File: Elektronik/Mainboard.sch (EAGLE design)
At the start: 21 parts

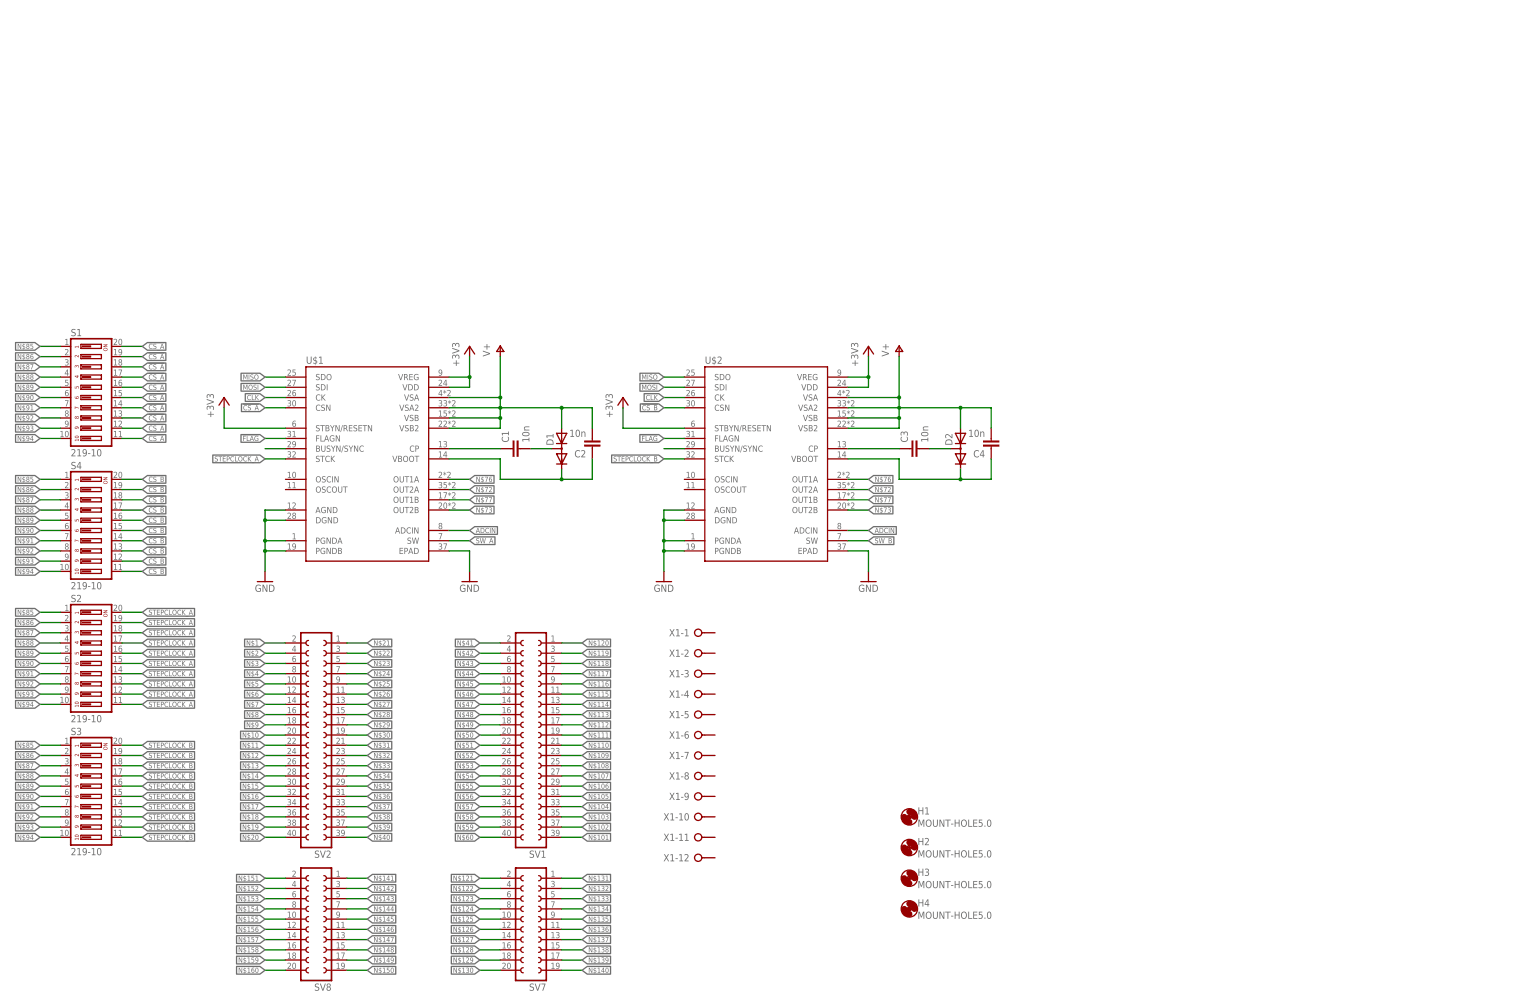
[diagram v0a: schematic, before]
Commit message: Elektronik auf den neusten Stand gebracht (Merge mit privater Dropbox
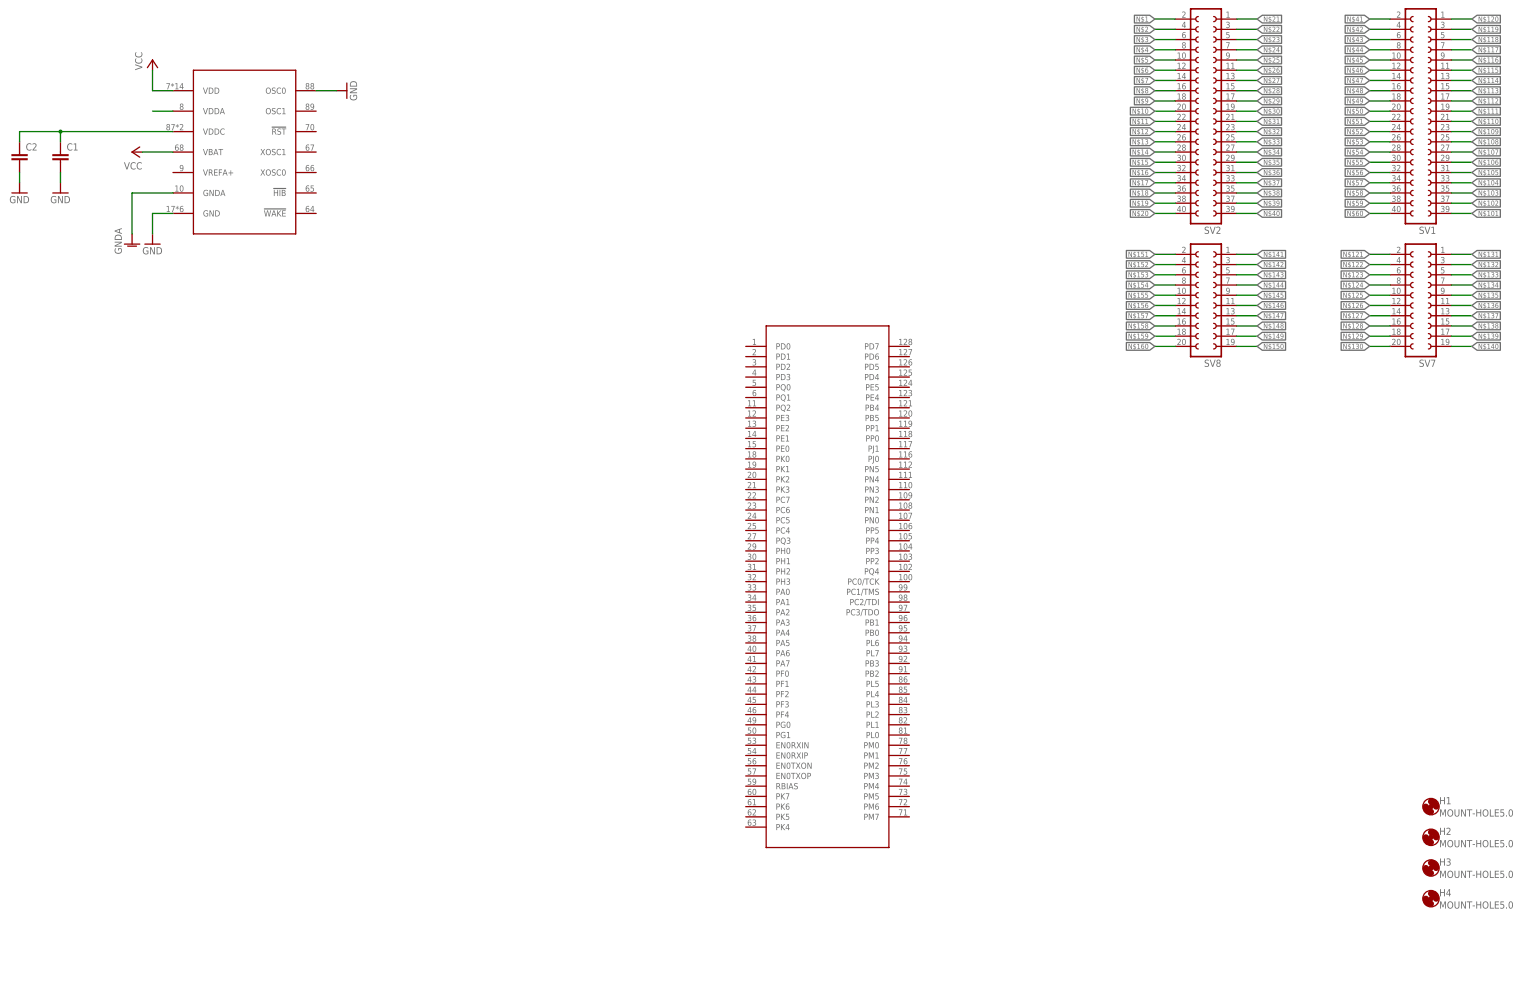
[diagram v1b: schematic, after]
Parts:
- removed C3, C4: 10n, rcl:C-EUC0805
- removed D1, D2: (no value), diode:DIODE_2CACA-SOT23
- removed S1, S2, S3, S4: 219-10, switch-dil:219-10
- removed U$2: L6470HPOWERSO36, Hardware:L6470HPOWERSO36
- removed X1: (no value), con-wago-508:W237-12P
- C1, C2: value 10n -> (none)
- U$1: value L6470HPOWERSO36 -> TM4C1294KCPDT; device Hardware:L6470HPOWERSO36 -> Hardware:TM4C1294KCPDT
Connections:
- removed net !CS_A: S1.11, S1.12, S1.13, S1.14, S1.15, S1.16, S1.17, S1.18, S1.19, S1.20, U$1.CSN
- removed net !CS_B: S4.11, S4.12, S4.13, S4.14, S4.15, S4.16, S4.17, S4.18, S4.19, S4.20, U$2.CSN
- removed net !FLAG: U$1.FLAGN, U$2.FLAGN
- removed net +3V3: U$1.STBYN/RESETN, U$1.VDD, U$1.VREG, U$2.STBYN/RESETN, U$2.VDD, U$2.VREG
- removed net ADCIN: U$1.ADCIN, U$2.ADCIN
- removed net CLK: U$1.CK, U$2.CK
- removed net MISO: U$1.SDO, U$2.SDO
- removed net MOSI: U$1.SDI, U$2.SDI
- removed net N$61: C3.1, U$2.CP
- removed net N$62: C3.2, D2.AC
- removed net N$63: C4.1, D2.C, U$2.VBOOT
- removed net N$67: U$1.BUSYN/SYNC, U$2.BUSYN/SYNC
- removed net N$71: C1.1, U$1.CP
- removed net N$72: U$1.OUT2A, U$2.OUT2A
- removed net N$73: U$1.OUT2B, U$2.OUT2B
- removed net N$74: C1.2, D1.AC
- removed net N$75: C2.1, D1.C, U$1.VBOOT
- removed net N$76: U$1.OUT1A, U$2.OUT1A
- removed net N$77: U$1.OUT1B, U$2.OUT1B
- removed net N$85: S1.1, S2.1, S3.1, S4.1
- removed net N$86: S1.2, S2.2, S3.2, S4.2
- removed net N$87: S1.3, S2.3, S3.3, S4.3
- removed net N$88: S1.4, S2.4, S3.4, S4.4
- removed net N$89: S1.5, S2.5, S3.5, S4.5
- removed net N$90: S1.6, S2.6, S3.6, S4.6
- removed net N$91: S1.7, S2.7, S3.7, S4.7
- removed net N$92: S1.8, S2.8, S3.8, S4.8
- removed net N$93: S1.9, S2.9, S3.9, S4.9
- removed net N$94: S1.10, S2.10, S3.10, S4.10
- removed net STEPCLOCK_A: S2.11, S2.12, S2.13, S2.14, S2.15, S2.16, S2.17, S2.18, S2.19, S2.20, U$1.STCK
- removed net STEPCLOCK_B: S3.11, S3.12, S3.13, S3.14, S3.15, S3.16, S3.17, S3.18, S3.19, S3.20, U$2.STCK
- removed net SW_A: U$1.SW
- removed net SW_B: U$2.SW
- removed net V+: C2.2, C4.2, D1.A, D2.A, U$1.VSA, U$1.VSA2, U$1.VSB, U$1.VSB2, U$2.VSA, U$2.VSA2, U$2.VSB, U$2.VSB2
- new net GNDA: U$1G$2.GNDA
- new net VCC: U$1G$2.VBAT, U$1G$2.VDD
- new net VDDA: U$1G$2.VDDA
- new net VDDC: C1.1, C2.1, U$1G$2.VDDC
- net GND: now also C1.2, C2.2, U$1G$2.GND, U$1G$2.OSC0; no longer U$1.AGND, U$1.DGND, U$1.EPAD, U$1.PGNDA, U$1.PGNDB, U$2.AGND, U$2.DGND, U$2.EPAD, U$2.PGNDA, U$2.PGNDB
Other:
- moved on the sheet: C1, C2, H1, H2, H3, H4, SV1, SV2, SV7, SV8
